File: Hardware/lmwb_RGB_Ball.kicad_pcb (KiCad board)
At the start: 2 copper layers, 65 x 65 mm, 30 parts, among them J1 Barrel_Jack_MountingPin, U1 24C02S, U2 AMS1117-3.3, U3 STM32C011F6P6

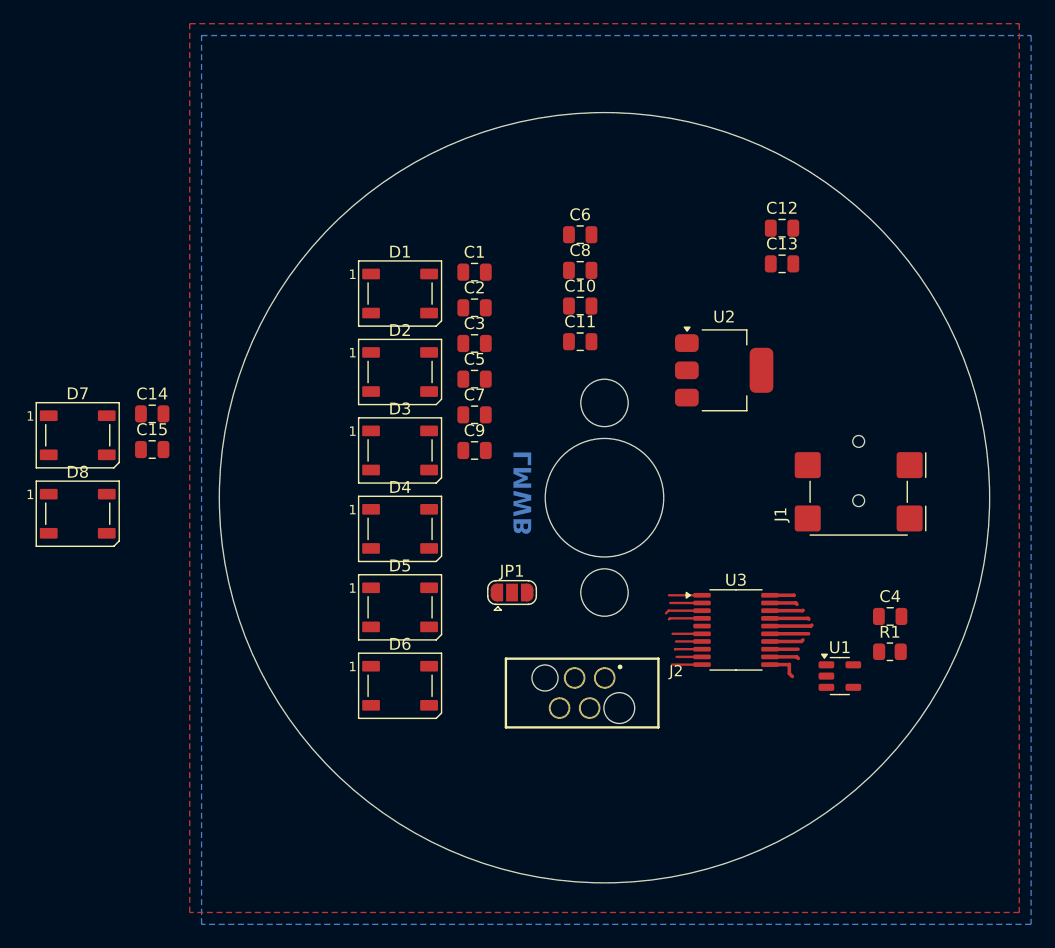
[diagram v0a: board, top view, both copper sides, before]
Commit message: did some routing
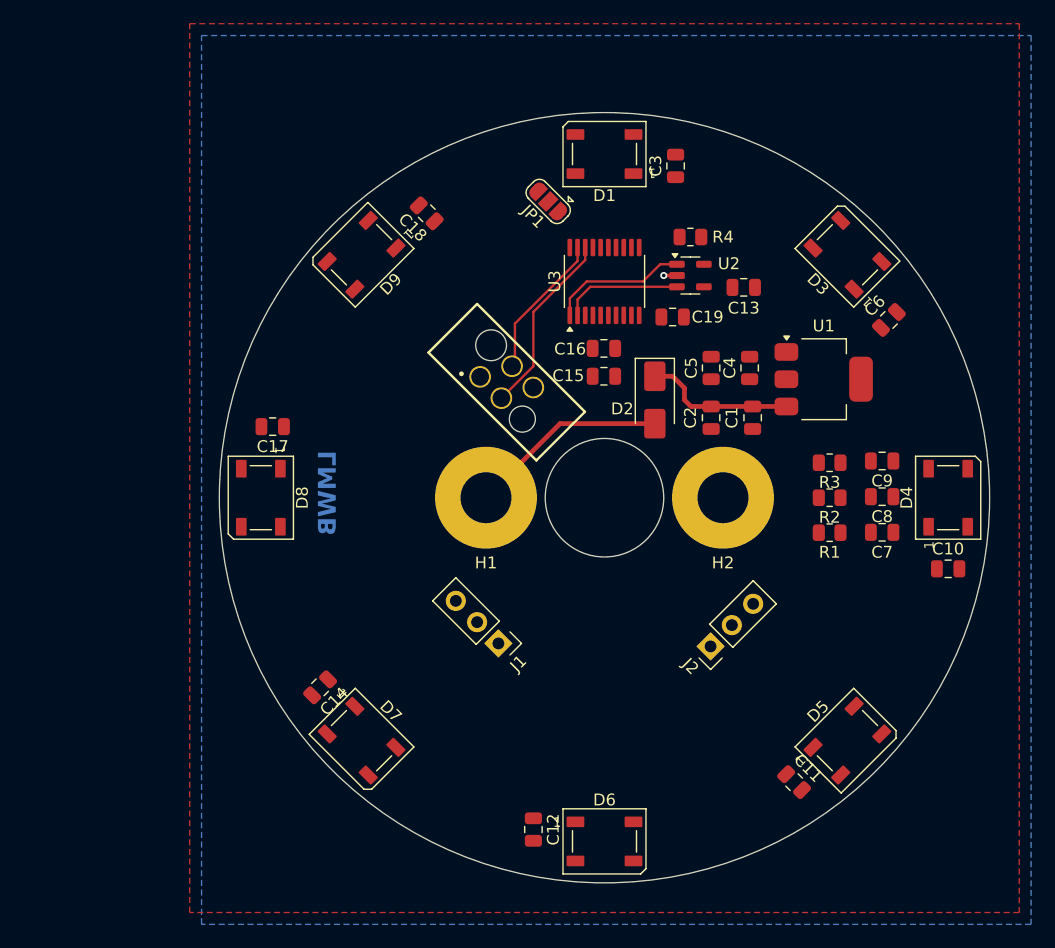
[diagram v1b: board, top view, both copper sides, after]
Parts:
- removed the C13 at (85.0, 50.3)
- added C16: 22u, Capacitor_SMD:C_0805_2012Metric, F.Cu at (70.0, 57.4)
- added C19: 100n, Capacitor_SMD:C_0805_2012Metric, F.Cu at (75.8, 54.8)
- added C7: 100n, Capacitor_SMD:C_0805_2012Metric, F.Cu at (93.4, 72.9)
- added C8: 100n, Capacitor_SMD:C_0805_2012Metric, F.Cu at (93.4, 69.9)
- added C9: 100n, Capacitor_SMD:C_0805_2012Metric, F.Cu at (93.4, 66.9)
- added D2: US1D, Diode_SMD:D_SMA, F.Cu at (74.2, 61.8)
- added H1: MountingHole_Pad, MountingHole:MountingHole_4.3mm_M4_Pad, F.Cu at (60.0, 70.0)
- added H2: MountingHole_Pad, MountingHole:MountingHole_4.3mm_M4_Pad, F.Cu at (80.0, 70.0)
- added J2: Conn_01x03, Connector_PinHeader_2.54mm:PinHeader_1x03_P2.54mm_Vertical, F.Cu at (79.0, 82.5)
- added R1: 10k, Resistor_SMD:R_0805_2012Metric, F.Cu at (89.0, 73.0)
- added R2: 10k, Resistor_SMD:R_0805_2012Metric, F.Cu at (89.0, 70.0)
- added R3: 10k, Resistor_SMD:R_0805_2012Metric, F.Cu at (89.0, 67.0)
- J1: value Barrel_Jack_MountingPin -> Conn_01x03; footprint Connector_BarrelJack:BarrelJack_Wuerth_694102107102_1.0x3.9mm -> Connector_PinHeader_2.54mm:PinHeader_1x03_P2.54mm_Vertical
- moved D4 46.4 mm to (99.0, 70.0), turned to 90 degrees
- moved C10 44.3 mm to (99.0, 76.0)
- moved C11 43.4 mm to (86.0, 94.0), turned to -45 degrees
- moved D5 41.8 mm to (90.5, 90.5), turned to 45 degrees
- moved D3 39.0 mm to (90.5, 49.5), turned to 135 degrees
- moved R4 38.8 mm to (77.2, 48.0)
- moved U2 36.1 mm to (77.2, 51.2)
- moved C12 35.3 mm to (64.0, 98.0), turned to -90 degrees
- moved C6 35.0 mm to (94.0, 55.0), turned to 45 degrees
- moved J1 33.4 mm to (61.0, 82.3), turned to -135 degrees
- moved JP1 33.1 mm to (65.2, 45.0), turned to 135 degrees
- moved D9 32.4 mm to (49.5, 49.5), turned to -135 degrees
- moved U3 31.4 mm to (70.0, 51.8), turned to 90 degrees
- moved C18 30.6 mm to (55.0, 46.0), turned to 135 degrees
- moved C13 30.4 mm to (81.8, 52.2)
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- renumbered C6 to C1, C3 to C10, C5 to C11, C7 to C12, C4 to C13, C9 to C14, C12 to C15, C14 to C17, C15 to C18, C8 to C2, C1 to C3, C10 to C4, C11 to C5, C2 to C6, D2 to D3, D3 to D4, D4 to D5, D5 to D6, D6 to D7, D7 to D8, D8 to D9, J2 to J3, R1 to R4, U2 to U1, U1 to U2
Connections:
- J1 pad 1: unconnected-(J1-Pad1) -> Net-(J1-Pin_1)
- J1 pad 2: unconnected-(J1-Pad2) -> Net-(J1-Pin_2)
- J1 pad 3: (no net) -> Net-(J1-Pin_3)
- J3 pad 1: unconnected-(J2-Pad1) -> GND
- J3 pad 2: unconnected-(J2-Pad2) -> /SW-CLK
- J3 pad 3: unconnected-(J2-Pad3) -> /SW-DIO
- J3 pad 4: unconnected-(J2-Pad4) -> +3V3
- JP1 pad 1: unconnected-(JP1-A-Pad1) -> /TIM1-CH1
- JP1 pad 3: unconnected-(JP1-B-Pad3) -> /SPI-MOSI
- U2 pad 1: unconnected-(U1-SCL-Pad1) -> /SCL
- U2 pad 3: unconnected-(U1-SDA-Pad3) -> /SDA
- U3 pad 1: unconnected-(U3-PB7-Pad1) -> /SCL
- U3 pad 11: unconnected-(U3-PA4-Pad11) -> /EXTI-4
- U3 pad 12: unconnected-(U3-PA5-Pad12) -> /EXTI-5
- U3 pad 13: unconnected-(U3-PA6-Pad13) -> /EXTI-6
- U3 pad 15: unconnected-(U3-PA8-Pad15) -> /TIM1-CH1
- U3 pad 17: unconnected-(U3-PA12-Pad17) -> /SPI-MOSI
- U3 pad 18: unconnected-(U3-PA13-Pad18) -> /SW-DIO
- U3 pad 19: unconnected-(U3-PA14-Pad19) -> /SW-CLK
- U3 pad 2: unconnected-(U3-PC14-Pad2) -> /SDA
- U3 pad 20: unconnected-(U3-PB6-Pad20) -> /SPI-SCK
- U3 pad 6: unconnected-(U3-PF2-Pad6) -> /nRST
- U3 pad 7: unconnected-(U3-PA0-Pad7) -> /UART-TX
- U3 pad 8: unconnected-(U3-PA1-Pad8) -> /UART-RX
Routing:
- net Net-(D2-A): track 0.00 -> 16.8 mm
- net /SW-DIO: track 0.00 -> 15.6 mm
- net VCC: track 0.00 -> 12.7 mm
- net /SW-CLK: track 0.00 -> 12.3 mm
- net /SCL: track 0.00 -> 11.7 mm
- net /SDA: track 0.00 -> 10.2 mm
- net unconnected-(U3-PA11-Pad16): track 3.58 -> 0.00 mm
- net unconnected-(U3-PA12-Pad17): track 3.32 -> 0.00 mm
- net unconnected-(U3-PA8-Pad15): track 3.28 -> 0.00 mm
- net unconnected-(U3-PC15-Pad3): track 3.14 -> 0.00 mm
- net unconnected-(U3-PA7-Pad14): track 2.85 -> 0.00 mm
- net +3V3: track 2.83 -> 0.00 mm
- net unconnected-(U3-PA13-Pad18): track 2.81 -> 0.00 mm
- net unconnected-(U3-PB7-Pad1): track 2.79 -> 0.00 mm
- net unconnected-(U3-PA4-Pad11): track 2.77 -> 0.00 mm
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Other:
- outline, holes or cut-outs redrawn
